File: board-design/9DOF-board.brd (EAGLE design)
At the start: 100 x 80 mm, 0 parts

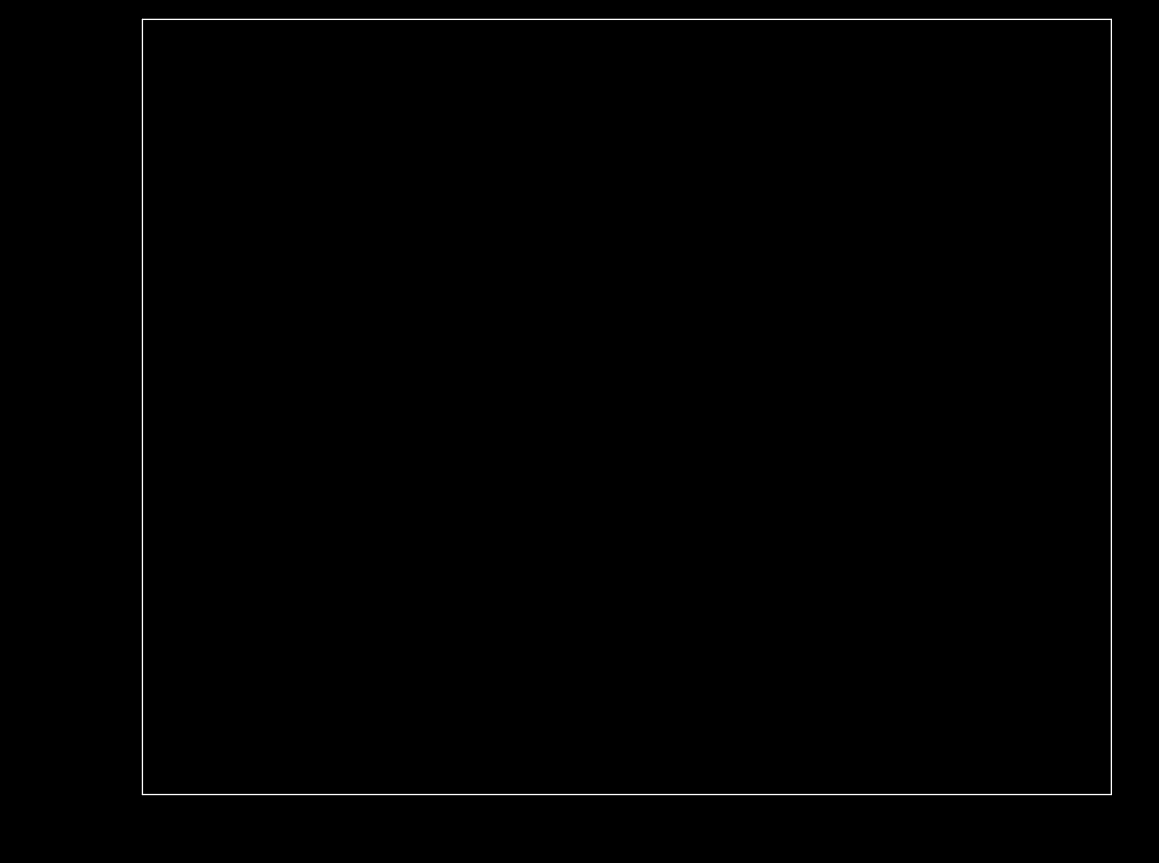
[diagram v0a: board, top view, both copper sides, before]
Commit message: Add files via upload
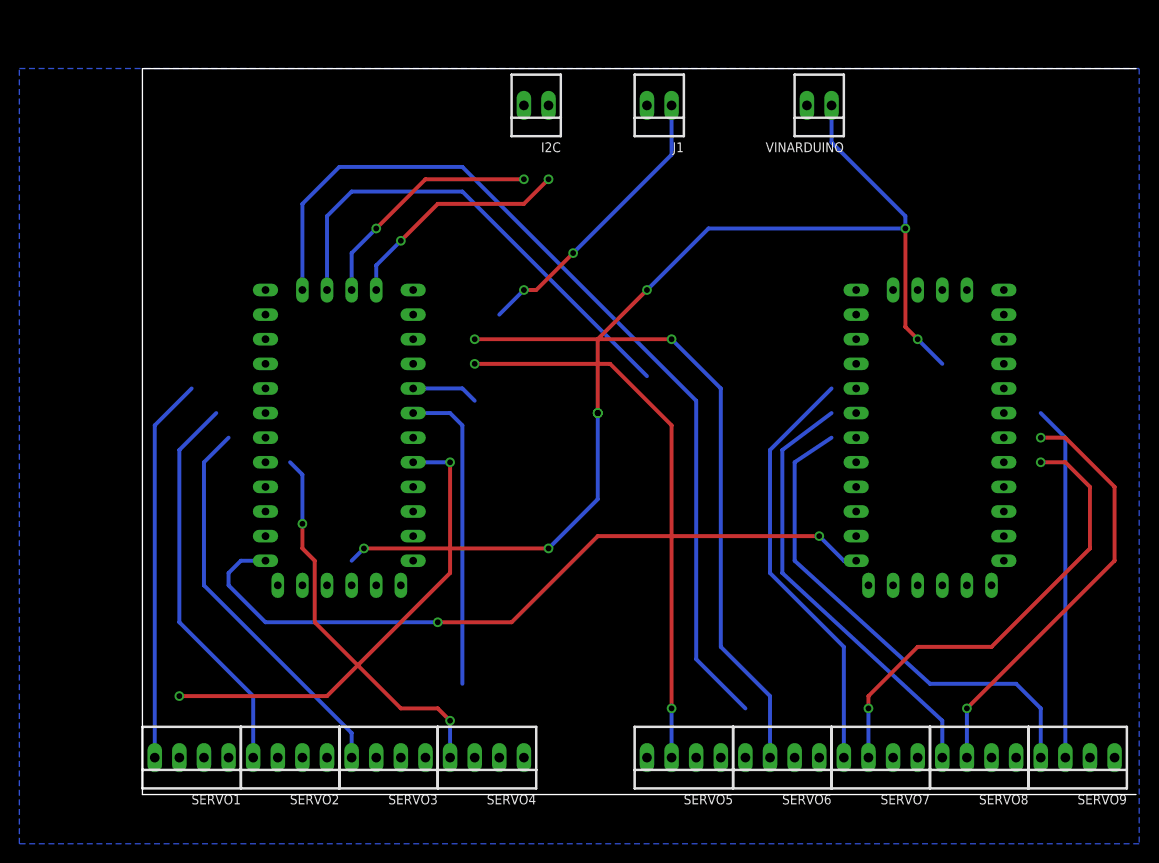
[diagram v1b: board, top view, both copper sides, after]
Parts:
- added I2C, J1, VINARDUINO: (no value), con-molex:22-23-2021
- added SERVO1, SERVO2, SERVO3, SERVO4, SERVO5, SERVO6, SERVO7, SERVO8, SERVO9: 22-23-2041, con-molex:22-23-2041
- added U$1, U$2: PRO-MINI, Arduino-clone:PRO-MINI
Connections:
- new net GND: J1.2, SERVO1.1, SERVO2.1, SERVO3.1, SERVO4.1, SERVO6.1, SERVO7.1, SERVO8.1, SERVO9.1, U$1.GND, U$1.GND2, U$1.GND3, U$2.GND, U$2.GND2, U$2.GND3, VINARDUINO.2
- new net I2C_SCL: I2C.2, U$1.A5
- new net I2C_SDA: I2C.1, U$1.A4
- new net RAW: U$1.RAW, U$2.RAW
- new net SERVO1_POT: SERVO1.4, U$1.A0
- new net SERVO1_SIG: SERVO1.3, U$1.D2
- new net SERVO2_POT: SERVO2.4, U$1.A1
- new net SERVO2_SIG: SERVO2.3, U$1.D3
- new net SERVO3_POT: SERVO3.4, U$1.A2
- new net SERVO3_SIG: SERVO3.3, U$1.D4
- new net SERVO4_POT: SERVO4.4, U$1.A3
- new net SERVO4_SIG: SERVO4.3, U$1.D5
- new net SERVO5_POT: SERVO5.4, U$1.A6
- new net SERVO5_SIG: SERVO5.3, U$1.D6
- new net SERVO6_POT: SERVO6.4, U$1.A7
- new net SERVO6_SIG: SERVO6.3, U$1.D7
- new net SERVO7_POT: SERVO7.4, U$2.A0
- new net SERVO7_SIG: SERVO7.3, U$2.D2
- new net SERVO8_POT: SERVO8.4, U$2.A1
- new net SERVO8_SIG: SERVO8.3, U$2.D3
- new net SERVO9_POT: SERVO9.4, U$2.A2
- new net SERVO9_SIG: SERVO9.3, U$2.D4
- new net VCC_ARDUINO: U$1.VCC1, U$2.VCC1, VINARDUINO.1
- new net VCC_SERVO: J1.1, SERVO1.2, SERVO2.2, SERVO3.2, SERVO4.2, SERVO5.2, SERVO6.2, SERVO7.2, SERVO8.2, SERVO9.2
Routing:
- net VCC_ARDUINO: track 0.00 -> 112.4 mm, vias 0 -> 8
- net SERVO6_POT: track 0.00 -> 95.0 mm
- net RAW: track 0.00 -> 76.7 mm, vias 0 -> 2
- net SERVO6_SIG: track 0.00 -> 67.7 mm, vias 0 -> 2
- net SERVO5_SIG: track 0.00 -> 57.2 mm, vias 0 -> 2
- net SERVO9_POT: track 0.00 -> 51.2 mm
- net SERVO5_POT: track 0.00 -> 49.6 mm
- net SERVO1_SIG: track 0.00 -> 48.4 mm, vias 0 -> 2
- net SERVO7_SIG: track 0.00 -> 48.0 mm, vias 0 -> 2
- net SERVO8_POT: track 0.00 -> 45.3 mm
- net SERVO8_SIG: track 0.00 -> 44.0 mm, vias 0 -> 2
- net SERVO7_POT: track 0.00 -> 43.9 mm
- net SERVO3_POT: track 0.00 -> 40.4 mm
- net SERVO2_POT: track 0.00 -> 40.3 mm
- net SERVO1_POT: track 0.00 -> 39.7 mm
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- added copper zone on layer 16, net GND
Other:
- board size 100 x 80 mm -> 102.5 x 74.9 mm
